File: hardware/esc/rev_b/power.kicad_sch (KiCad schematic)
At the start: 35 parts, among them J701 AUX_BATTERY, J702 FLIGHT_CAN_POWER, U701 LM5164DDA, U702 AP2112K-3.3TRG1, U703 LM5164DDA

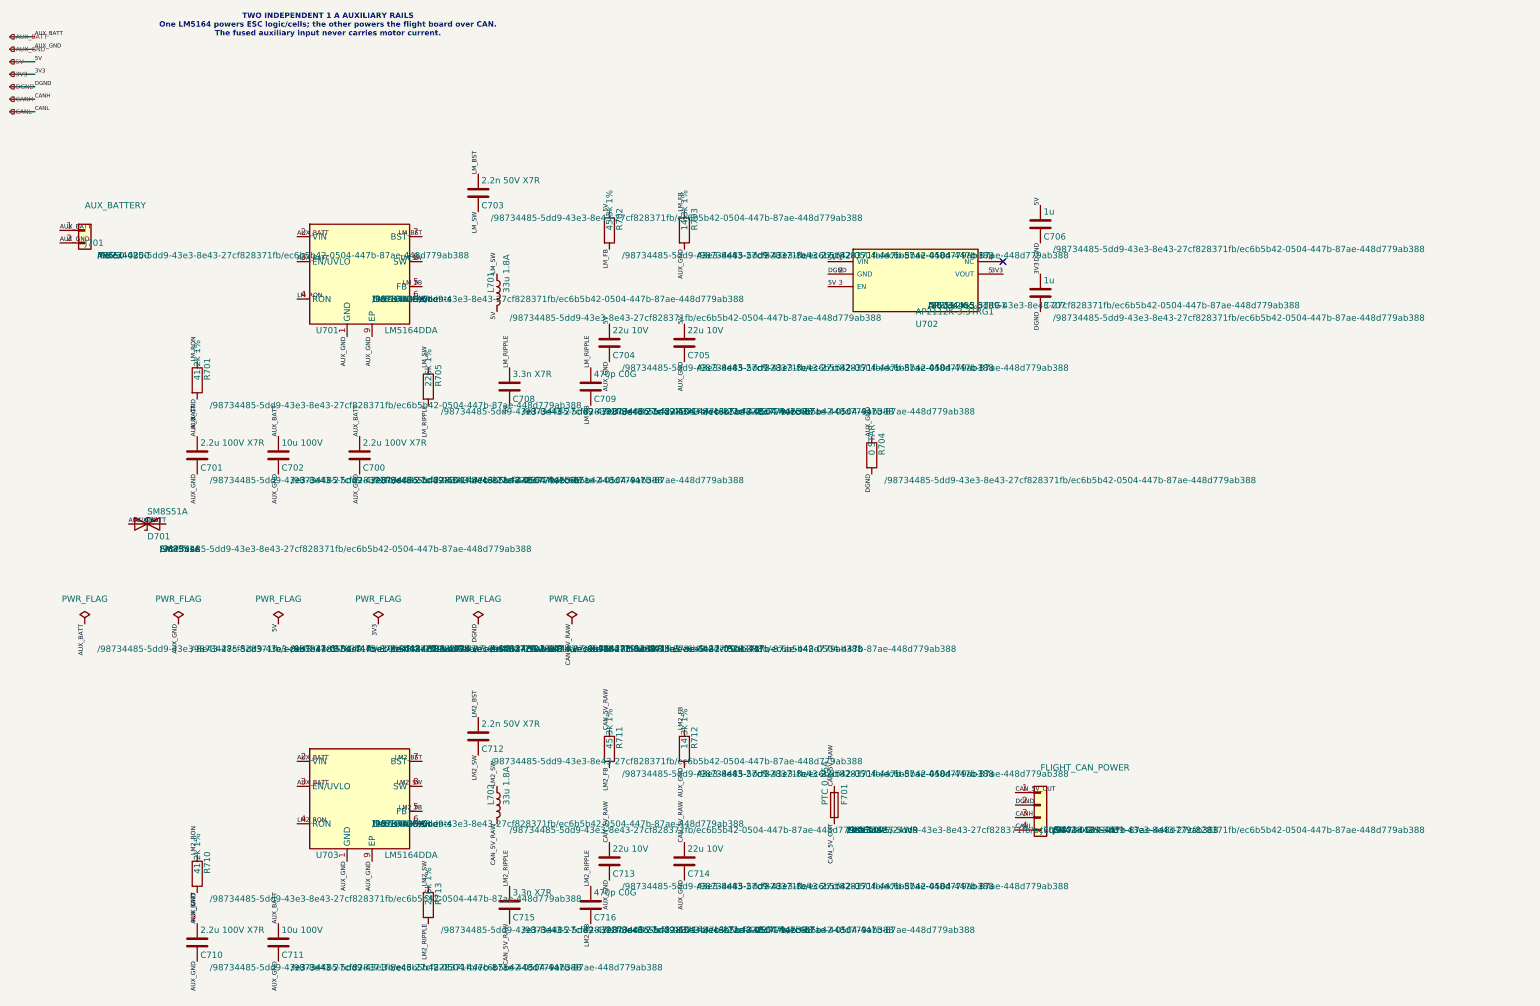
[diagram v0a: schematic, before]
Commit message: build: generate rev-b outputs
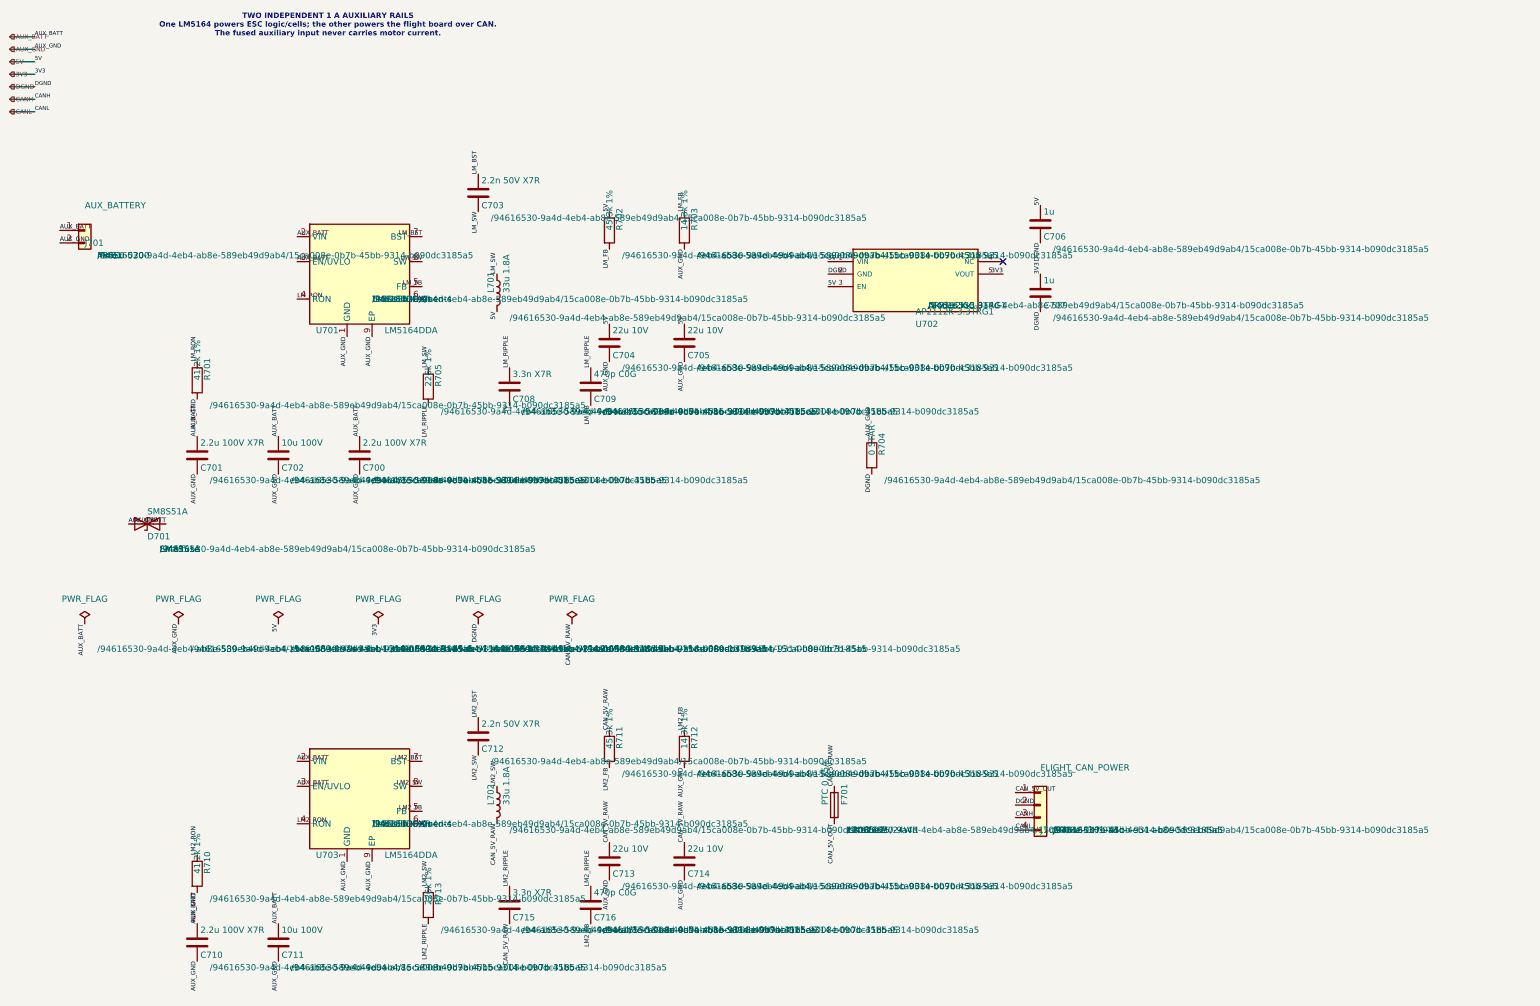
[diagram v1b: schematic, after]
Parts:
- C700, C701, C702, C703, C704, C705, C706, C707, C708, C709, C710, C711, C712, C713, C714, C715, C716, D701, F701, J701, J702, L701, L702, R701, R702, R703, R704, R705, R710, R711, R712, R713, U701, U702, U703: hierarchy_path /98734485-5dd9-43e3-8e43-27cf828371fb/ec6b5b42-0504-447b-87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 -> /94616530-9a4d-4eb4-ab8e-589eb49d9ab4/15ca008e-0b7b-45bb-93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
